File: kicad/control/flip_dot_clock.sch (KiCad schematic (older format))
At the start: 5 parts, among them U2 NCV7719

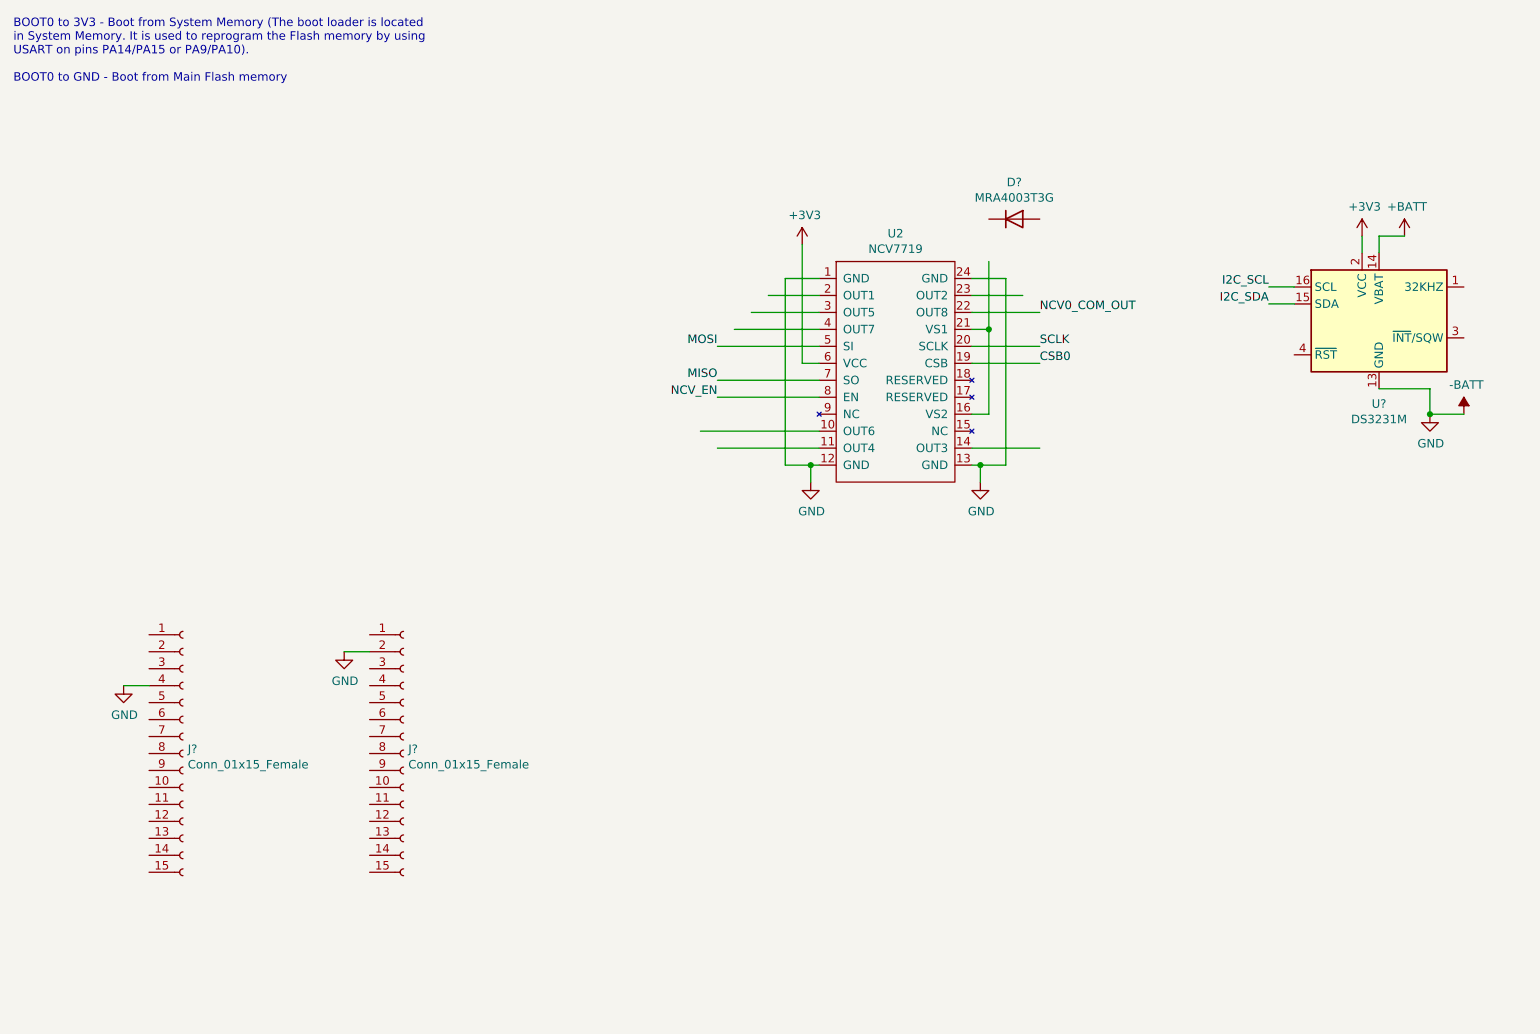
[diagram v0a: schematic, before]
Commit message: update schem
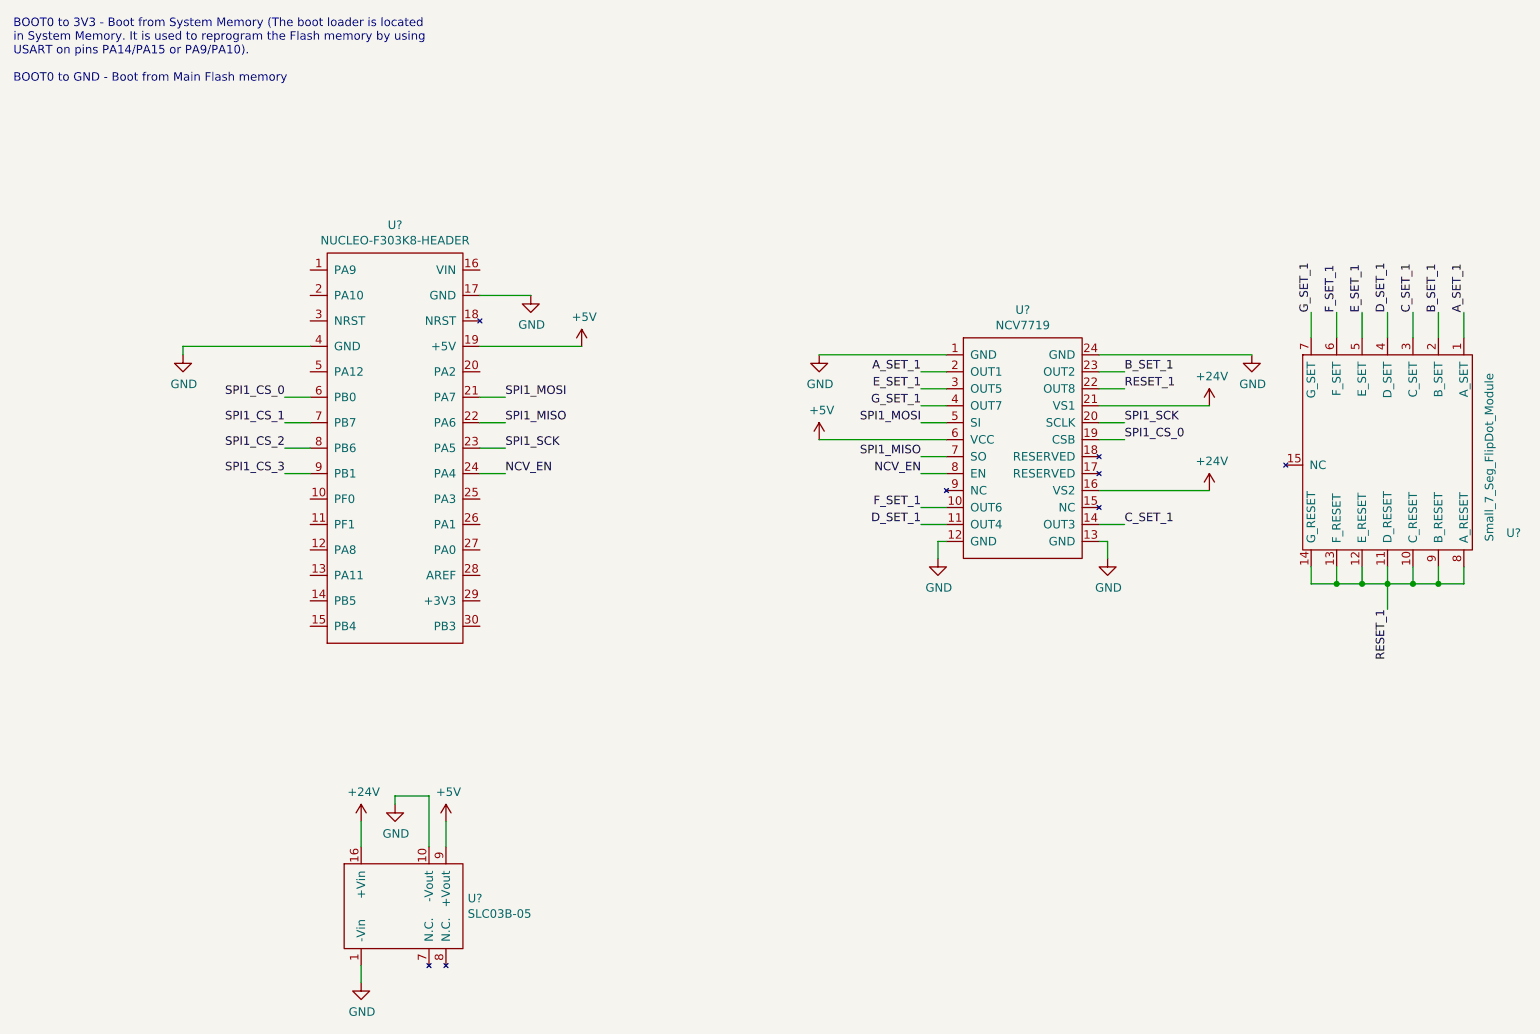
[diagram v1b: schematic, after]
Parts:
- removed D?: MRA4003T3G, Diode_SMD:D_SMA, symbol Diode:MRA4003T3G
- removed J? (x2): Conn_01x15_Female, symbol Connector:Conn_01x15_Female
- removed U2: NCV7719, mio:SSOP-24_6.4x7.55mm_P0.65mm, symbol flip_dot_clock-rescue:NCV7719-mio
- removed U?: DS3231M, Package_SO:SOIC-16W_7.5x10.3mm_P1.27mm, symbol Timer_RTC:DS3231M
- added U?: NUCLEO-F303K8-HEADER, symbol mio:NUCLEO-F303K8-HEADER
- added U?: NCV7719, mio:SSOP-24_6.4x7.55mm_P0.65mm, symbol flip_dot_clock-rescue:NCV7719-mio
- added U?: Small_7_Seg_FlipDot_Module, symbol mio:Small_7_Seg_FlipDot_Module
- added U?: SLC03B-05, symbol mio:SLC03B-05
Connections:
- net labels added: +24V, +5V, A_SET_1, B_SET_1, C_SET_1, D_SET_1, E_SET_1, F_SET_1, G_SET_1, RESET_1, SPI1_CS_0, SPI1_CS_1, SPI1_CS_2, SPI1_CS_3, SPI1_MISO, SPI1_MOSI, SPI1_SCK
- net labels removed: +3V3, +BATT, -BATT, CSB0, I2C_SCL, I2C_SDA, MISO, MOSI, NCV0_COM_OUT, SCLK
- wire segments 39 -> 61
